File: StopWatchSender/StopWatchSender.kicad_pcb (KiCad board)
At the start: 2 copper layers, 7 parts, among them IC1 ArduinoProMini, J1 Conn_01x02_Male, J2 Conn_01x06, U1 NRF24L01

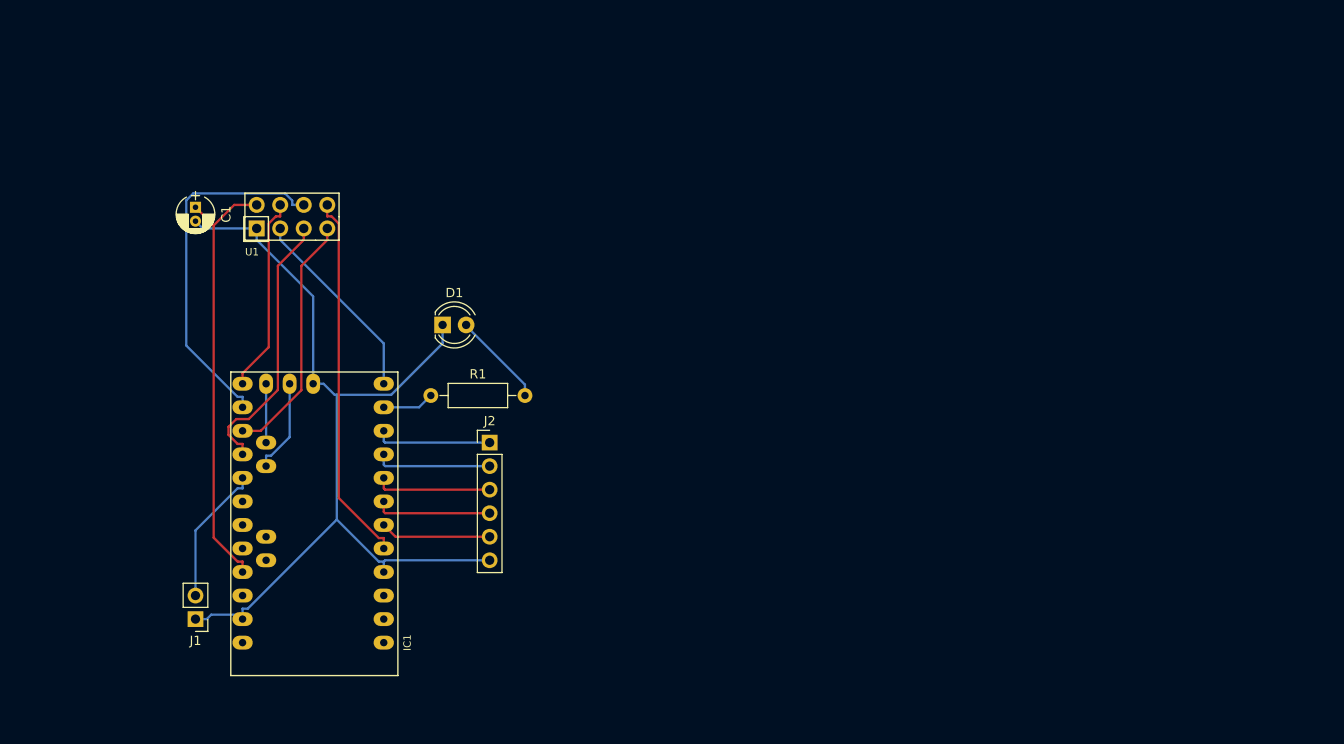
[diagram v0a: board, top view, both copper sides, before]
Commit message: wip
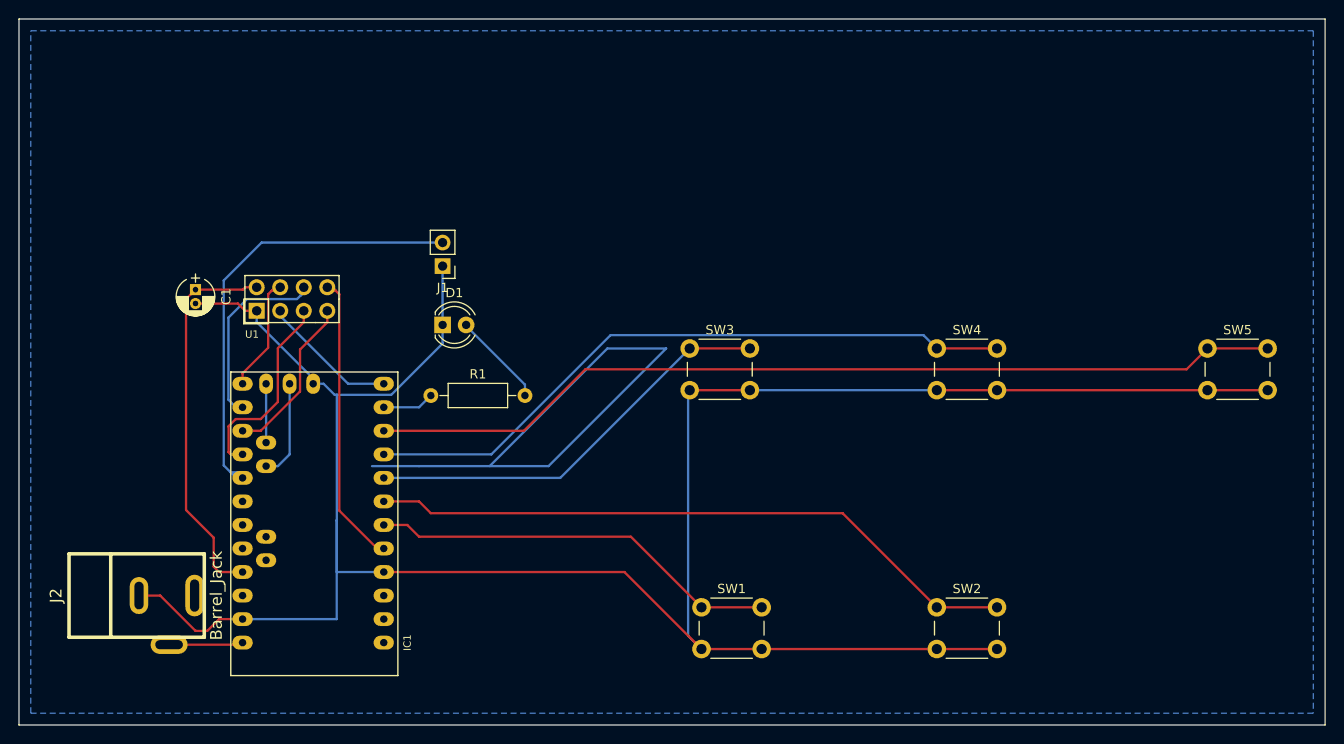
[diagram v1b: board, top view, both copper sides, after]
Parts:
- added SW1: SW_Push, Buttons_Switches_THT:SW_PUSH_6mm_h8mm, F.Cu at (147.3, 116.8)
- added SW2: SW_Push, Buttons_Switches_THT:SW_PUSH_6mm_h8mm, F.Cu at (172.7, 116.8)
- added SW3: SW_Push, Buttons_Switches_THT:SW_PUSH_6mm_h8mm, F.Cu at (146.1, 88.9)
- added SW4: SW_Push, Buttons_Switches_THT:SW_PUSH_6mm_h8mm, F.Cu at (172.7, 88.9)
- added SW5: SW_Push, Buttons_Switches_THT:SW_PUSH_6mm_h8mm, F.Cu at (201.9, 88.9)
- J2: value Conn_01x06 -> Barrel_Jack; footprint Pin_Headers:Pin_Header_Straight_1x06_Pitch2.54mm -> mysensors_connectors:dc_socket-kcswalter
- moved J1 46.5 mm to (119.4, 80.0)
- moved J2 41.5 mm to (86.4, 115.6), turned to 270 degrees
- moved C1 8.89 mm to (92.7, 82.5)
- moved U1 8.89 mm to (97.8, 86.4)
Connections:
- J2 pad 1: /PB_Start3 -> +5V
- J2 pad 2: /PB_Start2 -> GND
- J2 pad 3: /PB_Start1 -> Net-(J2-Pad3)
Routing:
- net GND: track 98.6 -> 323.4 mm
- net /PB_Start3: track 12.6 -> 99.1 mm
- net /PB_Start2: track 12.6 -> 72.1 mm
- net /PB_Start0: track 12.6 -> 70.9 mm
- net /Click_Amp: track 15.1 -> 48.9 mm
- net /PB_Start1: track 12.6 -> 45.3 mm
- net /PB_Stop: track 12.0 -> 44.5 mm
- net /nRF_MOSI: track 38.9 -> 21.2 mm
- net /nRF_MISO: track 26.8 -> 17.9 mm
- net /nRF_CSN: track 21.3 -> 13.0 mm
- net /nRF_IRQ: track 40.2 -> 32.1 mm
- net +5V: track 0.00 -> 8.02 mm
- net /nRF_SCK: track 29.5 -> 21.8 mm
- net /nRF_CE: track 21.4 -> 14.8 mm
- net /3.3V: track 47.3 -> 41.6 mm
- added copper zone on B.Cu, net GND
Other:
- board outline added: 141 x 76.2 mm
